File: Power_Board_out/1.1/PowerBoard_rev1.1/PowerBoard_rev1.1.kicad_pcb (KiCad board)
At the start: 4 copper layers, 40 x 40 mm, 31 parts, among them J1 HMTSW-102-X-X-S-X, J2 HMTSW-102-X-X-S-X, J3 HMTSW-102-X-X-S-X, J4 HMTSW-102-X-X-S-X, J5 HMTSW-102-X-X-S-X, J6 HMTSW-102-X-X-S-X, J7 530470210, J8 530470210, U1 DRV8410PWPR, U2 MCP73812T-420I-OT, U3 MCP73812T-420I-OT

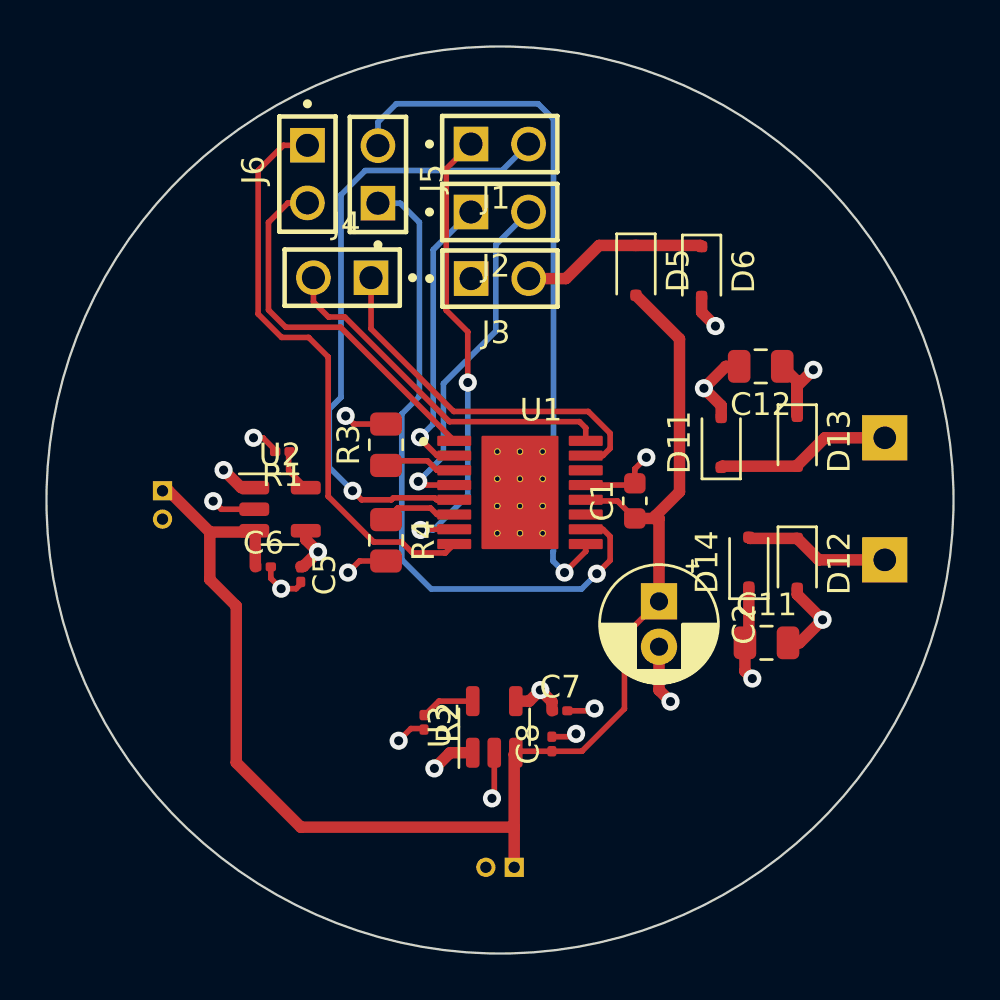
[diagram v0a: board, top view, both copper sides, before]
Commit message: POE 1 passes
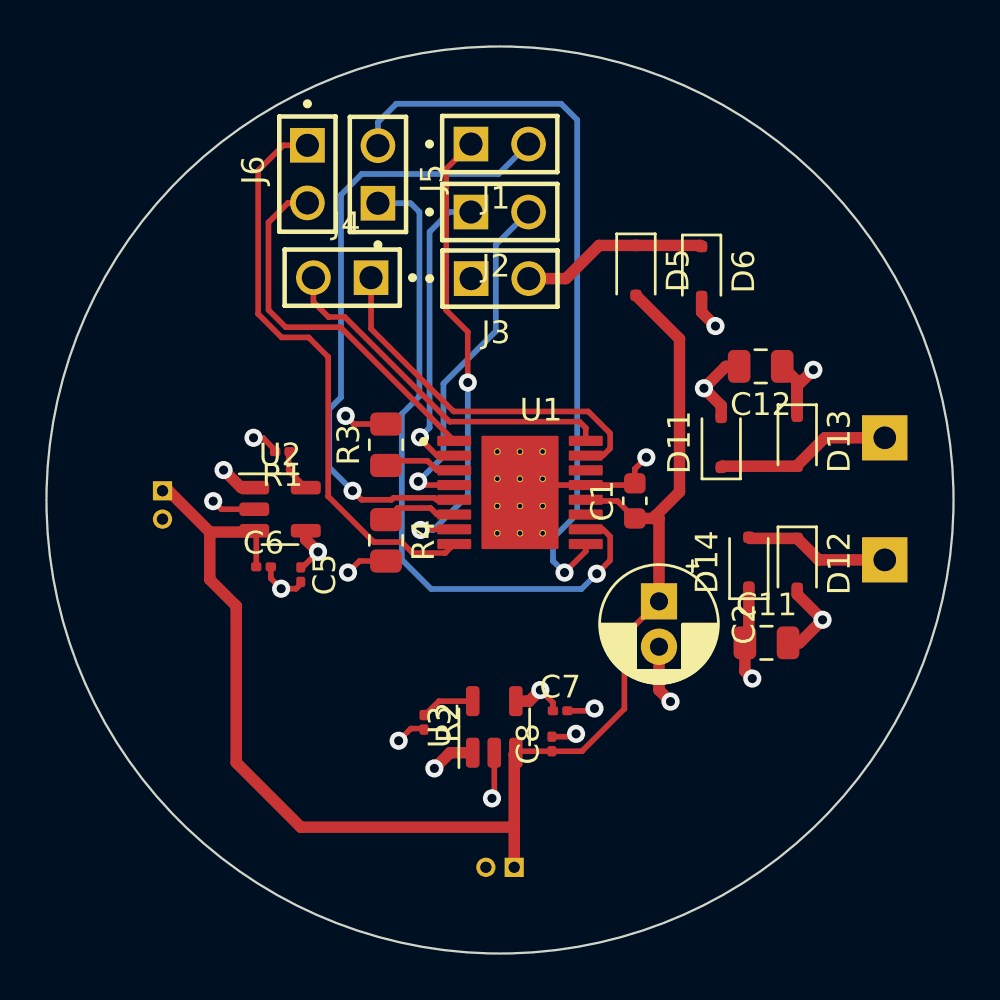
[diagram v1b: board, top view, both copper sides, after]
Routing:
- net GND: track 28.4 -> 31.5 mm
- net MOTOR2_BIN1: track 31.3 -> 32.7 mm
- net Net-(U1-AOUT1): track 12.7 -> 13.3 mm
